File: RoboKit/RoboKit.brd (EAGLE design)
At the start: 134 x 82 mm, 32 parts, among them CON1 XT30UPB-M, CON2 XT30UPB-M, P1 B6B-PH-K, P2 B6B-PH-K, U1 SSM6J808R, X3 JST-XH-02-PIN-LONG-PAD, X4 JST-XH-02-PIN-LONG-PAD, X5 JST-XH-04-PIN-LONG-PAD, X6 JST-XH-04-PIN-LONG-PAD, X7 JST-XH-10-PIN-LONG-PAD, X8 JST-XH-02-PIN-LONG-PAD, X9 JST-XH-03-PIN-LONG-PAD

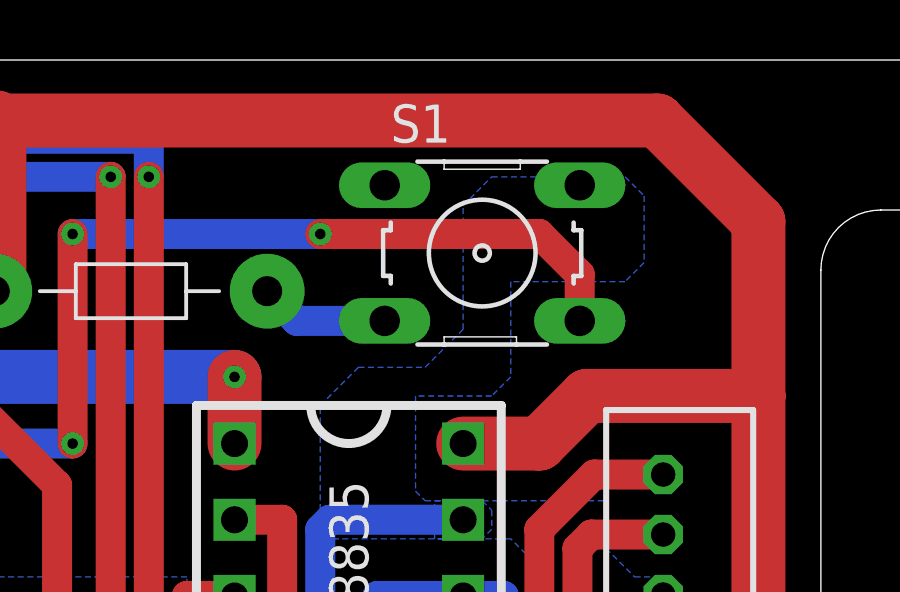
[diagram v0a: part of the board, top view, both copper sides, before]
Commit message: テスト8
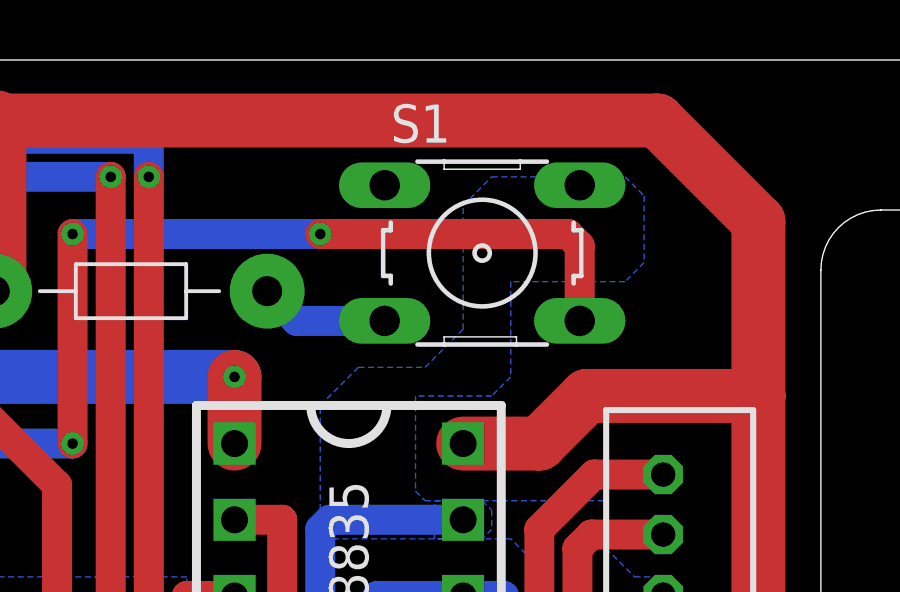
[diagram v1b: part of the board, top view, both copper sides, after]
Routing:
- net IO15: track 30.2 -> 30.7 mm
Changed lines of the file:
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@@
 <wire x1="87.3125" y1="76.2" x2="79.0575" y2="76.2" width="1" layer="16"/>
 <via x="87.3125" y="76.2" extent="1-16" drill="0.35"/>
-<wire x1="87.3125" y1="76.2" x2="94.615" y2="76.2" width="1" layer="1"/>
-<wire x1="95.9612" y1="74.8538" x2="95.9612" y2="73.3044" width="1" layer="1"/>
-<wire x1="94.615" y1="76.2" x2="95.9612" y2="74.8538" width="1" layer="1"/>
+<wire x1="87.3125" y1="76.2" x2="95.5675" y2="76.2" width="1" layer="1"/>
+<wire x1="95.9612" y1="75.8063" x2="95.9612" y2="73.3044" width="1" layer="1"/>
+<wire x1="95.5675" y1="76.2" x2="95.9612" y2="75.8063" width="1" layer="1"/>
 </signal>
 <signal name="VBUS" class="2">
